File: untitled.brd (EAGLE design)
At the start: 90 x 90 mm, 19 parts, among them X2 pzem-004t

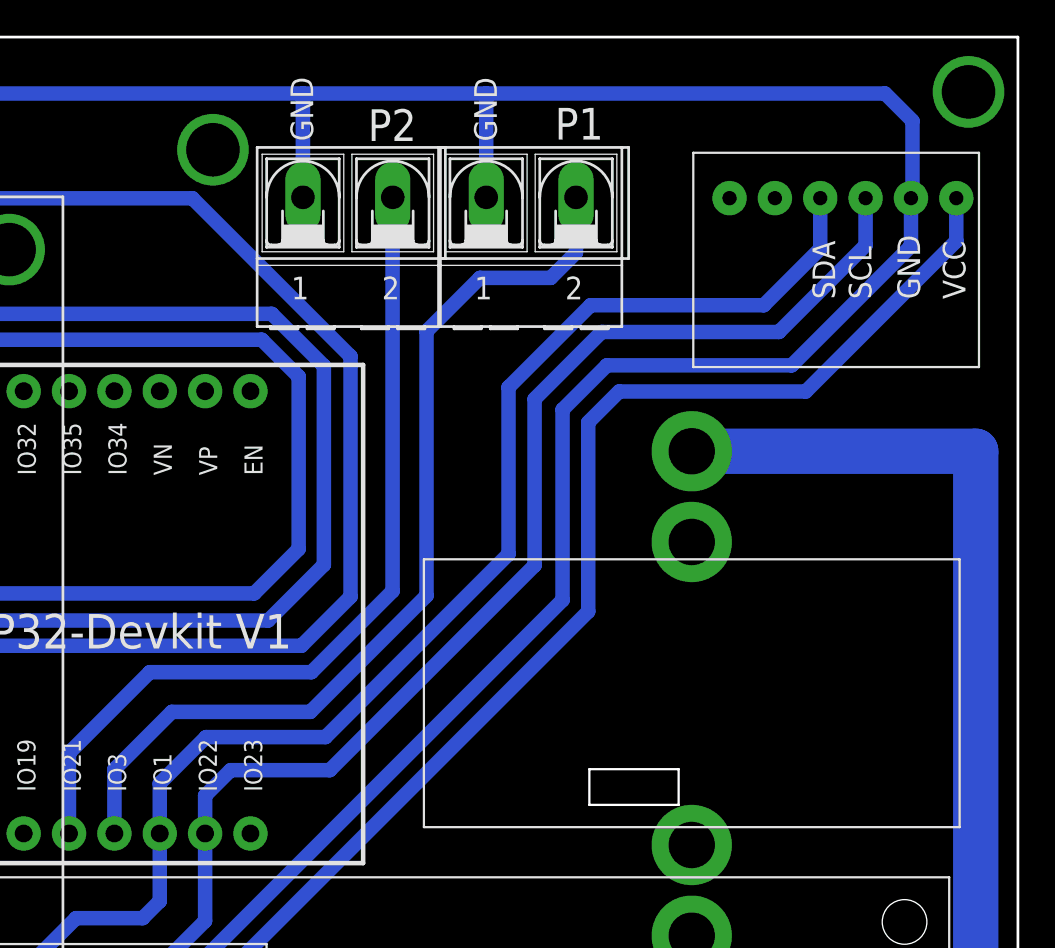
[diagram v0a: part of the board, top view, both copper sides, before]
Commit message: 213
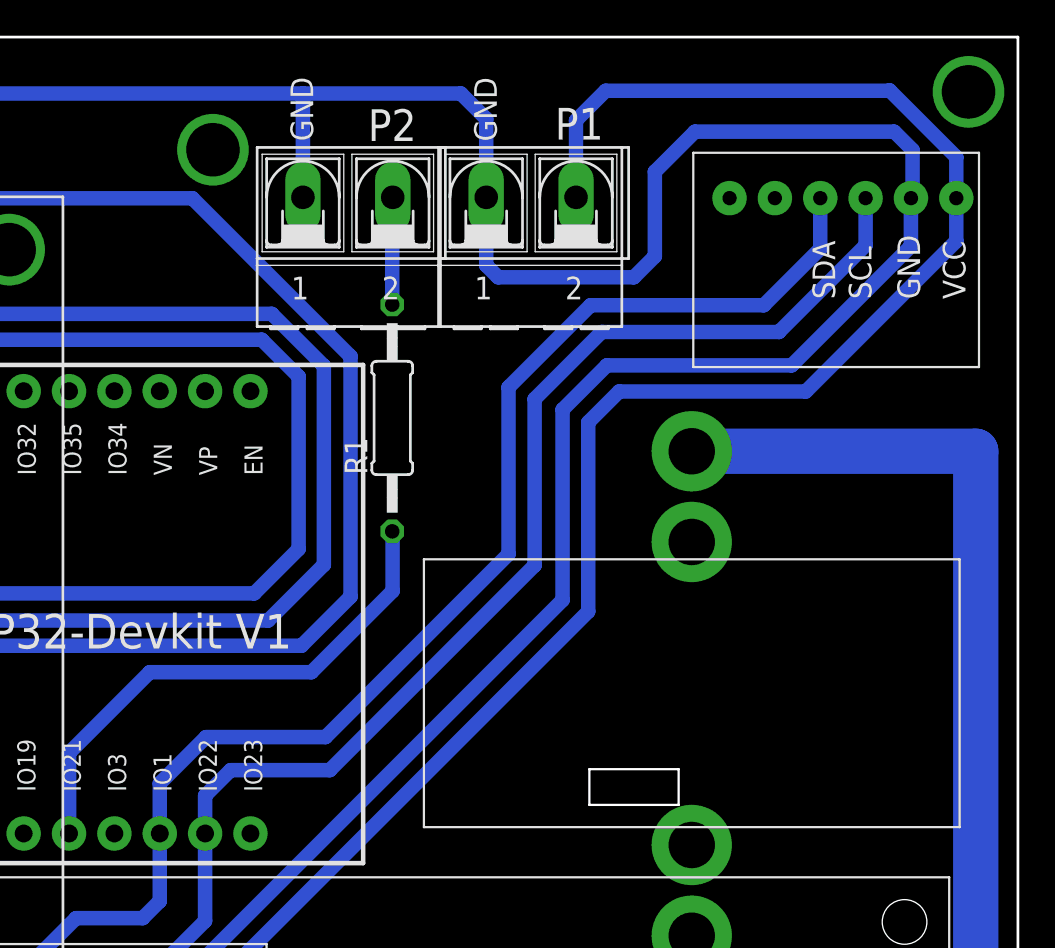
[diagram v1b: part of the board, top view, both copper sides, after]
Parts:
- added R1: 100, rcl:0207/12
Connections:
- new net N$1: P2.2, R1.2
- net D3: no longer P1.2
- net D4: now also R1.1; no longer P2.2
- net VCC: now also P1.2
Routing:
- net D3: track 53.2 -> 0.00 mm
- net VCC: track 209.6 -> 239.7 mm
- net D4: track 48.4 -> 29.7 mm
- net GND: track 246.2 -> 253.8 mm
- net N$1: track 0.00 -> 6.02 mm
